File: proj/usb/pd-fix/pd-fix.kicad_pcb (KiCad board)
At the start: 2 copper layers, 11 x 10 mm, 8 parts, among them J1 USB_C_Receptacle_USB2.0_16P, J2 Conn_01x02_Pin, U1 CH221K

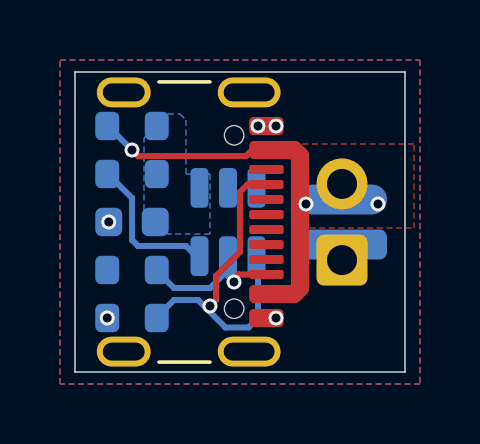
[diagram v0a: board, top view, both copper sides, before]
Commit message: -
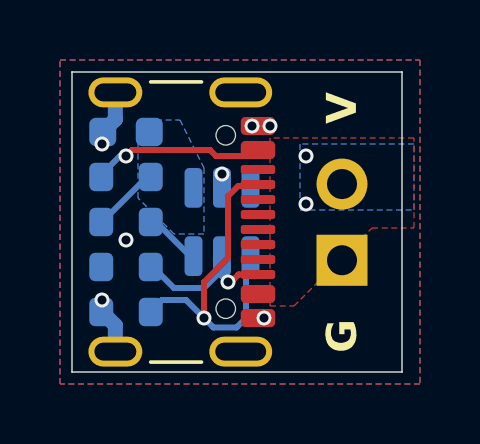
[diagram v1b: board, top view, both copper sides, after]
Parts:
- J2: footprint Library:SolderPad_2P -> Connector_PinHeader_2.54mm:PinHeader_1x02_P2.54mm_Vertical; moved to F.Cu
- moved C1 3.01 mm to (96.2, 97.0)
- moved R1 1.71 mm to (96.2, 98.5)
- moved R4 1.61 mm to (96.2, 100.0), turned to 0 degrees
- moved J2 1.28 mm to (103.4, 101.3), turned to 180 degrees
- moved R2 0.28 mm to (96.2, 103.0)
- moved J1 0.28 mm to (96.9, 100.0)
- moved R3 0.22 mm to (96.2, 101.5)
- moved U1 0.20 mm to (99.4, 100.0)
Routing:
- net VBUS: track 12.6 -> 5.81 mm
- net Net-(U1-CFG): track 5.03 -> 1.90 mm
- net GND: track 0.00 -> 2.88 mm, vias 5 -> 7
- net VDD: track 0.00 -> 2.22 mm
- added copper zone on B.Cu, net VBUS
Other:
- board text added: "12 473 15 104 20 204"
- board text added: "1u 1k ~0.28W CFG 4k7 4k7"
- board text added: "5 103 9 203"
- board text added: "@Mcbe Eringi PD-fix"
- board text added: "CH221K"
- board text added: "G"
- board text added: "PCB. 6CA.ME"
- board text added: "USB 4105"
- board text added: "V"
- board text removed: "103 5 473 12 203 9 104 15 204 20"
- board text removed: "1k ~0.28W CFG 1u 4k7 4k7"
- board text removed: "@Mcbe Eringi"
- board text removed: "CH221K PD-FIX"
